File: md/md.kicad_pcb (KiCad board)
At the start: 2 copper layers, 62.2 x 62.2 mm, 58 parts, among them J1 CONTROLL, J2 OUTA, J3 OUTB, J4 PWR_INPUT+, J5 PWR_INPUT-, J6 PWR_INPUT+, J7 PWR_INPUT+, J8 PWR_INPUT+, J9 PWR_INPUT+, Q1 IRFB7437PBF, Q2 IRFB7437PBF, Q3 IRFB7437PBF, Q4 IRFB7437PBF, U1 74HC00, U2 TLP2105, U3 IR7184S, U4 IR7184S, U5 LM7812_TO220

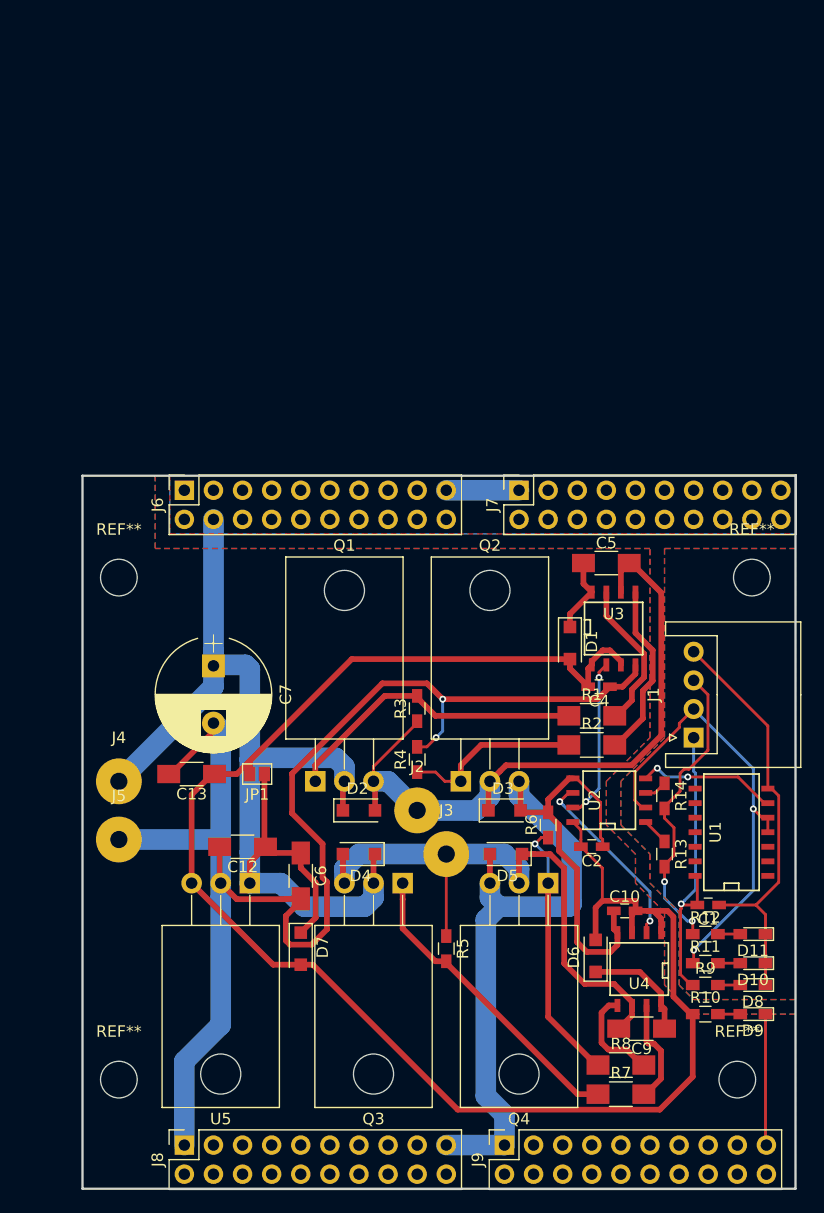
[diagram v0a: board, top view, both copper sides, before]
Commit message: PCBのガーバー出力
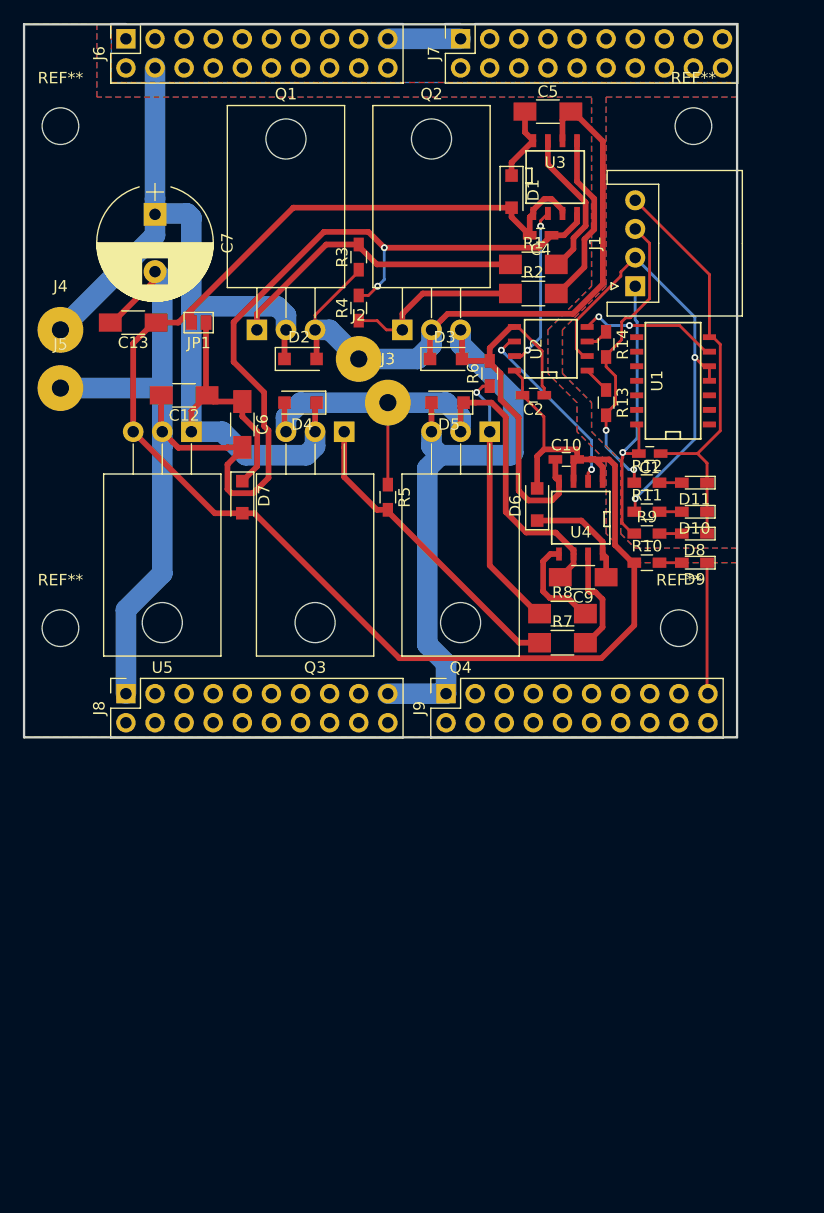
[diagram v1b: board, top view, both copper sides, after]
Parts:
- moved C10 39.7 mm to (47.3, 37.9)
- moved C13 39.7 mm to (9.51, 26.0)
- moved C2 39.7 mm to (44.4, 32.3)
- moved C7 39.7 mm to (11.4, 16.6)
- moved D1 39.7 mm to (42.5, 14.6)
- moved D10 39.7 mm to (58.5, 42.5)
- moved J4 39.7 mm to (3.15, 26.6)
- moved J5 39.7 mm to (3.15, 31.7)
- moved J8 39.7 mm to (8.87, 58.4)
- moved JP1 39.7 mm to (15.2, 26.0)
- moved Q2 39.7 mm to (33.0, 26.6)
- moved Q3 39.7 mm to (27.9, 35.5)
- moved Q4 39.7 mm to (40.6, 35.5)
- moved R1 39.7 mm to (44.4, 20.9)
- moved R14 39.7 mm to (50.8, 27.9)
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
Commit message: change regul
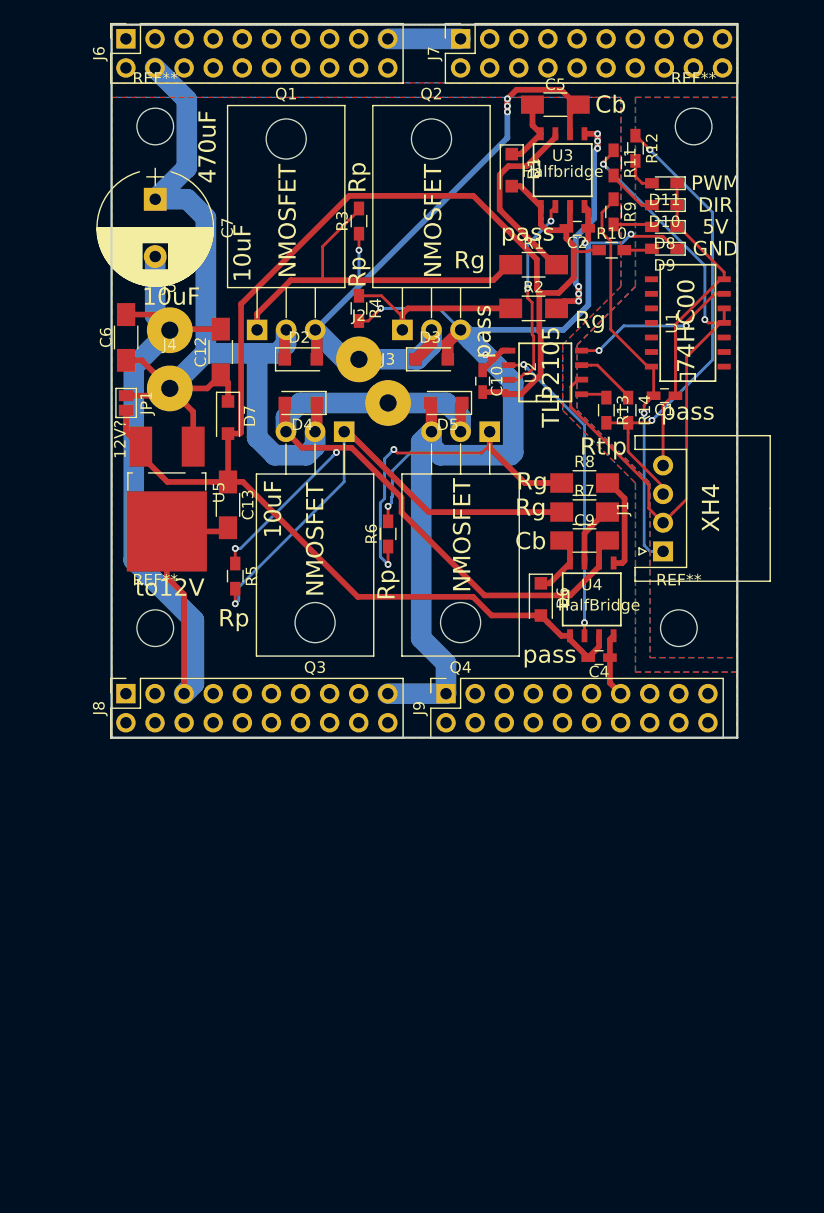
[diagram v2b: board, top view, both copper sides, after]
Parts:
- U5: footprint TO_SOT_Packages_THT:TO-220-3_Horizontal -> TO_SOT_Packages_SMD:TO-252-2_Rectifier
- moved C4 37.2 mm to (50.2, 55.2)
- moved R11 30.6 mm to (51.4, 12.1), turned to 270 degrees
- moved R12 29.2 mm to (53.3, 10.8), turned to 270 degrees
- moved R9 28.2 mm to (51.4, 16.3), turned to 270 degrees
- moved D9 27.5 mm to (55.9, 19.6)
- moved R10 27.4 mm to (51.3, 19.7)
- moved D10 26.9 mm to (55.9, 15.7)
- moved D8 26.9 mm to (55.9, 17.7)
- moved D11 26.3 mm to (55.9, 13.8)
- moved J1 23.3 mm to (55.8, 46.0)
- moved C13 17.9 mm to (17.8, 41.9), turned to 270 degrees
- moved R6 16.6 mm to (31.8, 44.5)
- moved C2 15.1 mm to (48.3, 17.8)
- moved R5 15.0 mm to (18.4, 48.1)
- moved C6 12.7 mm to (8.89, 27.3), turned to 90 degrees
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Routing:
- net GNDPWR: track 227.3 -> 186.7 mm, vias 2 -> 5
- net Net-(C9-Pad2): track 53.9 -> 75.6 mm, vias 0 -> 2
- net /DIR: track 40.7 -> 58.1 mm
- net Net-(Q3-Pad1): track 27.1 -> 42.1 mm, vias 0 -> 1
- net /PWM: track 26.4 -> 41.4 mm
- net +24V: track 104.4 -> 92.2 mm
- net /OUTB: track 16.3 -> 27.2 mm
- net +12V: track 147.3 -> 137.8 mm
- net GND: track 37.2 -> 28.9 mm
- net Net-(Q4-Pad1): track 23.0 -> 31.2 mm, vias 1 -> 2
- net +5V: track 26.8 -> 34.9 mm
- net Net-(R2-Pad2): track 15.4 -> 22.0 mm, vias 0 -> 6
- net Net-(C5-Pad2): track 60.8 -> 67.0 mm, vias 0 -> 4
- net Net-(Q1-Pad1): track 26.8 -> 32.9 mm
- net Net-(C9-Pad1): track 9.71 -> 5.55 mm
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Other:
- board size 62.2 x 62.2 mm -> 54.6 x 62.2 mm
- board text added: "10uF"
- board text added: "12V?"
- board text added: "24V"
- board text added: "470uF"
- board text added: "5V"
- board text added: "74HC00"
- board text added: "Cb"
- board text added: "DIR"
- board text added: "Designed by: Nakano Masaki"
- board text added: "FETTORCH v0.0.2"
- board text added: "GND"
- board text added: "HalfBridge"
- board text added: "Halfbridge"
- board text added: "NMOSFET"
- board text added: "National Institute of Techonlogy, Kagawa College, Takamatsu. Mechanical Research Club."
- board text added: "OUTA"
- board text added: "OUTB"
- board text added: "PWM"
- board text added: "Rg"
- board text added: "Rp"
- board text added: "Rtlp"
- board text added: "TLP2105"
- board text added: "Vcc"
- board text added: "XH4"
- board text added: "pass"
- board text added: "to12V"
